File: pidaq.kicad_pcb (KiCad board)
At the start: 2 copper layers, 83.8 x 78.1 mm, 42 parts, among them J1 Screw_Terminal_01x08, J2 Screw_Terminal_01x08, J3 Screw_Terminal_01x10, J4 Screw_Terminal_01x10, J5 Conn_01x03_Male, J6 Conn_01x08_Female, U1 LTC2984CLX-DNP, U2 LTC2418IGN-DNP, U3 SN74LV1T34DCKR

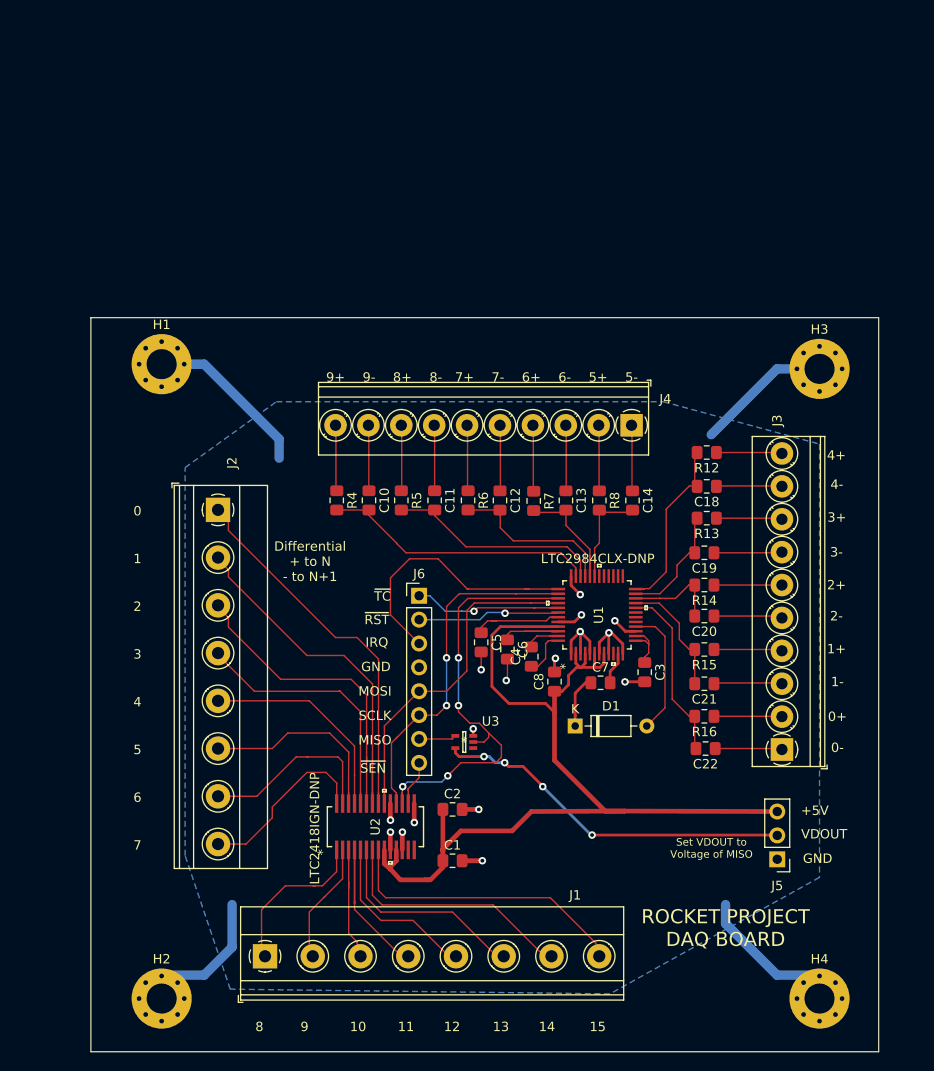
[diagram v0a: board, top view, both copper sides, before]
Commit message: completed design 2.0
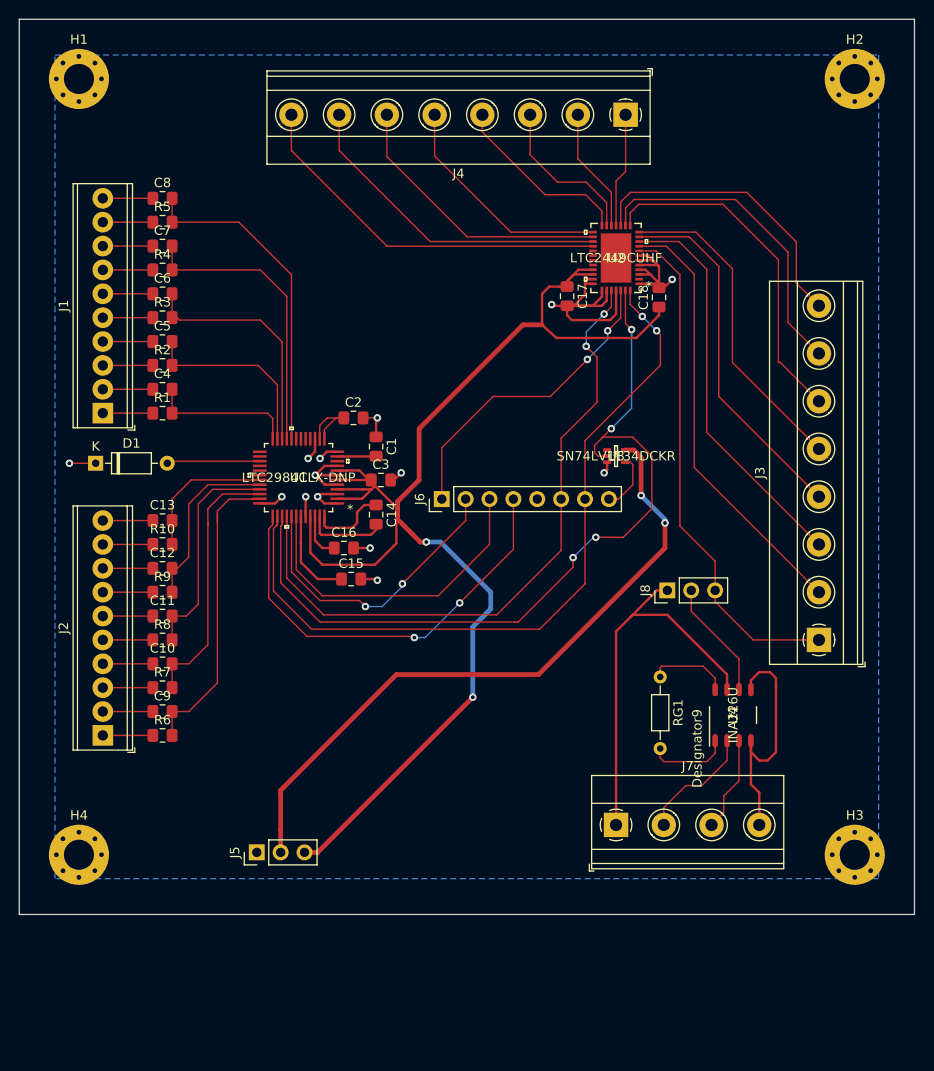
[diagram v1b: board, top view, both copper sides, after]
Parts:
- removed C19, C20, C21, C22: 100pF, Capacitor_SMD:C_0805_2012Metric_Pad1.15x1.40mm_HandSolder
- removed R12, R13, R14, R15, R16: 100, Resistor_SMD:R_0805_2012Metric_Pad1.15x1.40mm_HandSolder
- added C15: 10uF, Capacitor_SMD:C_0805_2012Metric_Pad1.15x1.40mm_HandSolder, F.Cu at (105.2, 110.4)
- added C16: 10uF, Capacitor_SMD:C_0805_2012Metric_Pad1.15x1.40mm_HandSolder, F.Cu at (104.4, 107.1)
- added C17: 10uF, Capacitor_SMD:C_0805_2012Metric_Pad1.15x1.40mm_HandSolder, F.Cu at (128.1, 80.3)
- added C9: 100pF, Capacitor_SMD:C_0805_2012Metric_Pad1.15x1.40mm_HandSolder, F.Cu at (85.1, 124.5)
- added J7: Screw_Terminal_01x04, TerminalBlock_Phoenix:TerminalBlock_Phoenix_MKDS-1,5-4-5.08_1x04_P5.08mm_Horizontal, F.Cu at (133.3, 136.5)
- added J8: Conn_01x03_Male, Connector_PinHeader_2.54mm:PinHeader_1x03_P2.54mm_Vertical, F.Cu at (138.8, 111.6)
- added R1: 100, Resistor_SMD:R_0805_2012Metric_Pad1.15x1.40mm_HandSolder, F.Cu at (85.1, 92.7)
- added R10: 100, Resistor_SMD:R_0805_2012Metric_Pad1.15x1.40mm_HandSolder, F.Cu at (85.1, 106.7)
- added R2: 100, Resistor_SMD:R_0805_2012Metric_Pad1.15x1.40mm_HandSolder, F.Cu at (85.1, 87.6)
- added R3: 100, Resistor_SMD:R_0805_2012Metric_Pad1.15x1.40mm_HandSolder, F.Cu at (85.1, 82.5)
- added R9: 100, Resistor_SMD:R_0805_2012Metric_Pad1.15x1.40mm_HandSolder, F.Cu at (85.1, 111.8)
- added RG1: R_US, Resistor_THT:R_Axial_DIN0204_L3.6mm_D1.6mm_P7.62mm_Horizontal, F.Cu at (138.0, 120.8)
- added U4: INA126U, footprints:INA126U, F.Cu at (145.8, 124.8)
- C1: value 10uF -> 100nF
- C14: value 100pF -> 10uF
- C18: value 100pF -> 0.1uF
- C2: value 100nF -> 1uF
- C3: value 1uF -> 100nF
- C4, C5, C6: value 10uF -> 100pF
- C7, C8: value 100nF -> 100pF
- J1, J2: value Screw_Terminal_01x08 -> Screw_Terminal_01x10; footprint TerminalBlock_Phoenix:TerminalBlock_Phoenix_MKDS-1,5-8-5.08_1x08_P5.08mm_Horizontal -> TerminalBlock_Phoenix:TerminalBlock_Phoenix_MPT-0,5-10-2.54_1x10_P2.54mm_Horizontal
- J3, J4: value Screw_Terminal_01x10 -> Screw_Terminal_01x08; footprint TerminalBlock_Phoenix:TerminalBlock_Phoenix_PT-1,5-10-3.5-H_1x10_P3.50mm_Horizontal -> TerminalBlock_Phoenix:TerminalBlock_Phoenix_MKDS-1,5-8-5.08_1x08_P5.08mm_Horizontal
- U1: footprint proj_footprints:LTC2984CLX-PBF -> footprints:LTC2984CLX-PBF
- U2: value LTC2418IGN-DNP -> LTC2449CUHF; footprint proj_footprints:LTC2418IGN-PBF -> footprints:LTC2449CUHF
- U3: footprint proj_footprints:SN74LV1T34DCKR -> footprints:SN74LV1T34DCKR
- moved H2 122.5 mm to (158.8, 57.1)
- moved H4 80.3 mm to (76.2, 139.7)
- moved C8 66.2 mm to (85.1, 69.8), turned to 0 degrees
- moved C7 65.8 mm to (85.1, 74.9)
- moved U2 65.7 mm to (133.3, 76.2), turned to 180 degrees
- moved J1 60.3 mm to (78.7, 92.7), turned to 90 degrees
- moved D1 58.2 mm to (78.0, 98.0)
- moved J5 55.4 mm to (95.1, 139.4), turned to 90 degrees
- moved C6 52.7 mm to (85.1, 80.0), turned to 0 degrees
- moved H3 51.8 mm to (158.8, 139.7)
- moved R8 48.8 mm to (85.1, 116.8), turned to 0 degrees
- moved C4 48.5 mm to (85.1, 90.2), turned to 0 degrees
- moved C5 46.6 mm to (85.1, 85.1), turned to 0 degrees
- moved C1 44.8 mm to (107.8, 96.3), turned to 270 degrees
- moved R7 44.2 mm to (85.1, 121.9), turned to 0 degrees
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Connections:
- C1 pad 1: +5V -> GND
- C1 pad 2: GND -> Net-(C1-Pad2)
- C10 pad 2: TC9+ -> TC8+
- C11 pad 2: TC8+ -> TC7+
- C12 pad 2: TC7+ -> TC6+
- C13 pad 2: TC6+ -> TC5+
- C14 pad 1: GND -> Net-(C14-Pad1)
- C14 pad 2: TC5+ -> Net-(C14-Pad2)
- C18 pad 1: GND -> +5V
- C18 pad 2: TC4+ -> GND
- C2 pad 1: +5V -> Net-(C2-Pad1)
- C3 pad 1: Net-(C3-Pad1) -> +5V
- C4 pad 1: Net-(C4-Pad1) -> GND
- C4 pad 2: Net-(C4-Pad2) -> TC4+
- C5 pad 1: Net-(C5-Pad1) -> GND
- C5 pad 2: GND -> TC3+
- C6 pad 1: Net-(C6-Pad1) -> GND
- C6 pad 2: GND -> TC2+
- C7 pad 2: Net-(C7-Pad2) -> TC1+
- C8 pad 1: +5V -> GND
- C8 pad 2: GND -> TC0+
- D1 pad 2: Net-(D1-Pad2) -> /thermocouples/CJ
- J1 pad 1: Net-(J1-Pad1) -> /thermocouples/TC4RAW
- J1 pad 2: Net-(J1-Pad2) -> GND
- J1 pad 3: Net-(J1-Pad3) -> /thermocouples/TC3RAQ
- J1 pad 4: Net-(J1-Pad4) -> GND
- J1 pad 5: Net-(J1-Pad5) -> /thermocouples/TC2RAW
- J1 pad 6: Net-(J1-Pad6) -> GND
- J1 pad 7: Net-(J1-Pad7) -> /thermocouples/TC1RAW
- J1 pad 8: Net-(J1-Pad8) -> GND
- J2 pad 1: /SEN0 -> /thermocouples/TC9RAW
- J2 pad 2: /SEN1 -> GND
- J2 pad 3: /SEN2 -> /thermocouples/TC8RAW
- J2 pad 4: /SEN3 -> GND
- J2 pad 5: /SEN4 -> /thermocouples/TC7RAW
- J2 pad 6: /SEN5 -> GND
- J2 pad 7: /SEN6 -> /thermocouples/TC6RAW
- J2 pad 8: /SEN7 -> GND
- J3 pad 1: GND -> SEN0
- J3 pad 2: Net-(J3-Pad2) -> SEN1
- J3 pad 3: GND -> SEN2
- J3 pad 4: Net-(J3-Pad4) -> SEN3
- J3 pad 5: GND -> SEN4
- J3 pad 6: Net-(J3-Pad6) -> SEN5
- J3 pad 7: GND -> SEN6
- J3 pad 8: Net-(J3-Pad8) -> SEN7
- J4 pad 1: GND -> SEN8
- J4 pad 2: Net-(J4-Pad2) -> SEN9
- J4 pad 3: GND -> SEN10
- J4 pad 4: Net-(J4-Pad4) -> SEN11
- J4 pad 5: GND -> SEN12
- J4 pad 6: Net-(J4-Pad6) -> SEN13
- J4 pad 7: GND -> SEN14
- J4 pad 8: Net-(J4-Pad8) -> SEN15
- J6 pad 1: ~TC -> ~SEN
- J6 pad 2: RST -> ~TC
- J6 pad 3: IRQ -> ~RST
- J6 pad 4: GND -> IRQ
- J6 pad 5: MOSI -> GND
- J6 pad 6: SCLK -> MOSI
- J6 pad 7: /MISO_SAFE -> SCLK
- J6 pad 8: ~SEN -> /MISO_SAFE
- R4 pad 1: Net-(J4-Pad10) -> /thermocouples/TC1RAW
- R4 pad 2: TC9+ -> TC1+
- R5 pad 1: Net-(J4-Pad8) -> /thermocouples/TC0RAW
- R5 pad 2: TC8+ -> TC0+
- R6 pad 1: Net-(J4-Pad6) -> /thermocouples/TC9RAW
- R6 pad 2: TC7+ -> TC9+
- R7 pad 1: Net-(J4-Pad4) -> /thermocouples/TC8RAW
- R7 pad 2: TC6+ -> TC8+
- R8 pad 1: Net-(J4-Pad2) -> /thermocouples/TC7RAW
- R8 pad 2: TC5+ -> TC7+
- U1 pad 11: Net-(C7-Pad2) -> Net-(C1-Pad2)
- U1 pad 13: Net-(C3-Pad1) -> Net-(C2-Pad1)
- U1 pad 14: Net-(C3-Pad1) -> Net-(C2-Pad1)
- U1 pad 16: Net-(D1-Pad2) -> (no net)
- U1 pad 27: (no net) -> /thermocouples/CJ
- U1 pad 42: RST -> ~RST
- U1 pad 43: Net-(C5-Pad1) -> Net-(C15-Pad1)
- U1 pad 46: Net-(C6-Pad1) -> Net-(C16-Pad1)
- U1 pad 47: Net-(C4-Pad2) -> Net-(C14-Pad2)
- U1 pad 48: Net-(C4-Pad1) -> Net-(C14-Pad1)
- U2 pad 1: Net-(J1-Pad1) -> GND
- U2 pad 10: GND -> SEN2
- U2 pad 11: +5V -> SEN3
- U2 pad 12: GND -> SEN4
- U2 pad 13: (no net) -> SEN5
- U2 pad 14: (no net) -> SEN6
- U2 pad 15: GND -> SEN7
- U2 pad 16: ~SEN -> SEN8
- U2 pad 17: MISO -> SEN9
- U2 pad 18: SCLK -> SEN10
- U2 pad 19: GND -> SEN11
- U2 pad 2: Net-(J1-Pad2) -> (no net)
- U2 pad 20: MOSI -> SEN12
- U2 pad 21: /SEN0 -> SEN13
- U2 pad 22: /SEN1 -> SEN14
- U2 pad 23: /SEN2 -> SEN15
- U2 pad 24: /SEN3 -> (no net)
- U2 pad 25: /SEN4 -> (no net)
- U2 pad 26: /SEN5 -> (no net)
- U2 pad 27: /SEN6 -> (no net)
- U2 pad 28: /SEN7 -> +5V
- U2 pad 3: Net-(J1-Pad3) -> GND
- U2 pad 4: Net-(J1-Pad4) -> GND
- U2 pad 5: Net-(J1-Pad5) -> GND
- U2 pad 6: Net-(J1-Pad6) -> GND
- U2 pad 7: Net-(J1-Pad7) -> GND
- U2 pad 8: Net-(J1-Pad8) -> SEN0
- U2 pad 9: +5V -> SEN1
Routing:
- net SEN0: track 0.00 -> 55.9 mm
- net SEN1: track 0.00 -> 46.4 mm
- net SCLK: track 37.5 -> 81.0 mm
- net SEN2: track 0.00 -> 42.6 mm
- net +EXC: track 0.00 -> 42.6 mm
- net /SEN0: track 41.5 -> 0.00 mm
- net MISO: track 46.0 -> 87.0 mm
- net /SEN1: track 41.0 -> 0.00 mm
- net SEN15: track 0.00 -> 40.1 mm
- net +5V: track 105.5 -> 144.2 mm, vias 0 -> 2
- net SEN3: track 0.00 -> 38.7 mm
- net SEN5: track 0.00 -> 36.9 mm
- net SEN14: track 0.00 -> 34.8 mm
- net SEN4: track 0.00 -> 34.5 mm
- net ~RST: track 0.00 -> 34.5 mm
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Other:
- board size 83.8 x 78.1 mm -> 95.2 x 95.3 mm
- board text removed: "+5V"
- board text removed: "0"
- board text removed: "0+"
- board text removed: "0-"
- board text removed: "1"
- board text removed: "1+"
- board text removed: "1-"
- board text removed: "10"
- board text removed: "11"
- board text removed: "12"
- board text removed: "13"
- board text removed: "14"
- board text removed: "15"
- board text removed: "2"
- board text removed: "2+"
- board text removed: "2-"
- board text removed: "3"
- board text removed: "3+"
- board text removed: "3-"
- board text removed: "4"
- board text removed: "4+"
- board text removed: "4-"
- board text removed: "5"
- board text removed: "5+"
- board text removed: "5-"
- board text removed: "6"
- board text removed: "6+"
- board text removed: "6-"
- board text removed: "7"
- board text removed: "7+"
- board text removed: "7-"
- board text removed: "8"
- board text removed: "8+"
- board text removed: "8-"
- board text removed: "9"
- board text removed: "9+"
- board text removed: "9-"
- board text removed: "Differential + to N - to N+1"
- board text removed: "GND"
- board text removed: "IRQ"
- board text removed: "MISO"
- board text removed: "MOSI"
- board text removed: "ROCKET PROJECT DAQ BOARD"
- board text removed: "SCLK"
- board text removed: "Set VDOUT to Voltage of MISO"
- board text removed: "VDOUT"
- board text removed: "~RST"
- board text removed: "~SEN"
- board text removed: "~TC"
